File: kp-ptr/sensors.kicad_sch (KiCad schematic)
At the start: 3 parts

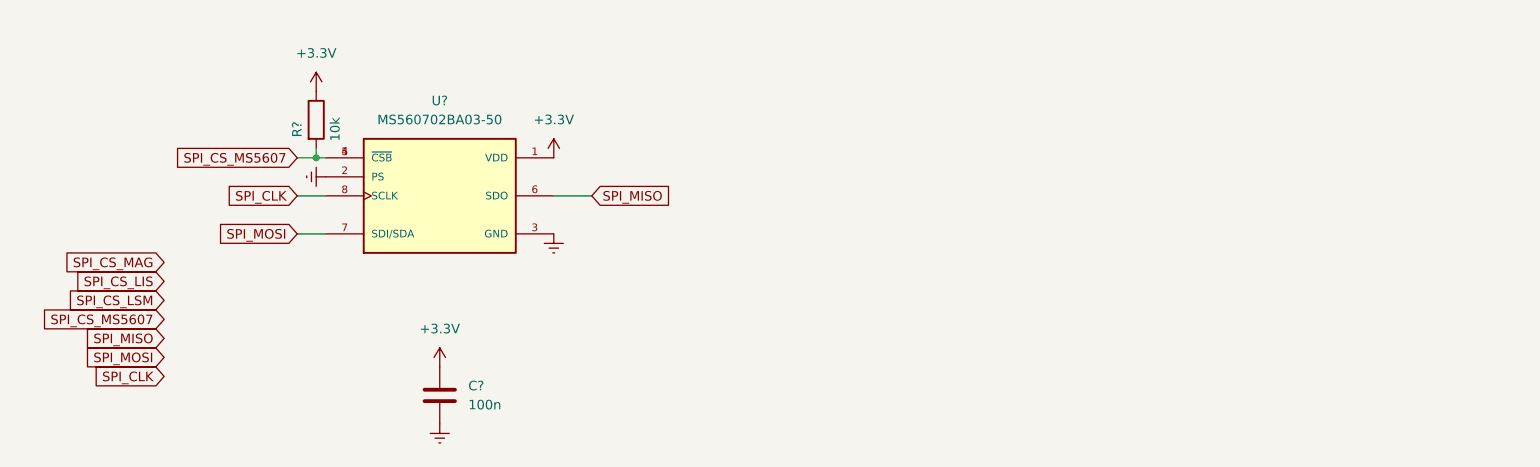
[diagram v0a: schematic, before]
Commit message: LIS + SDCARD Signed-off-by: kretu <krecik@gmail.com>
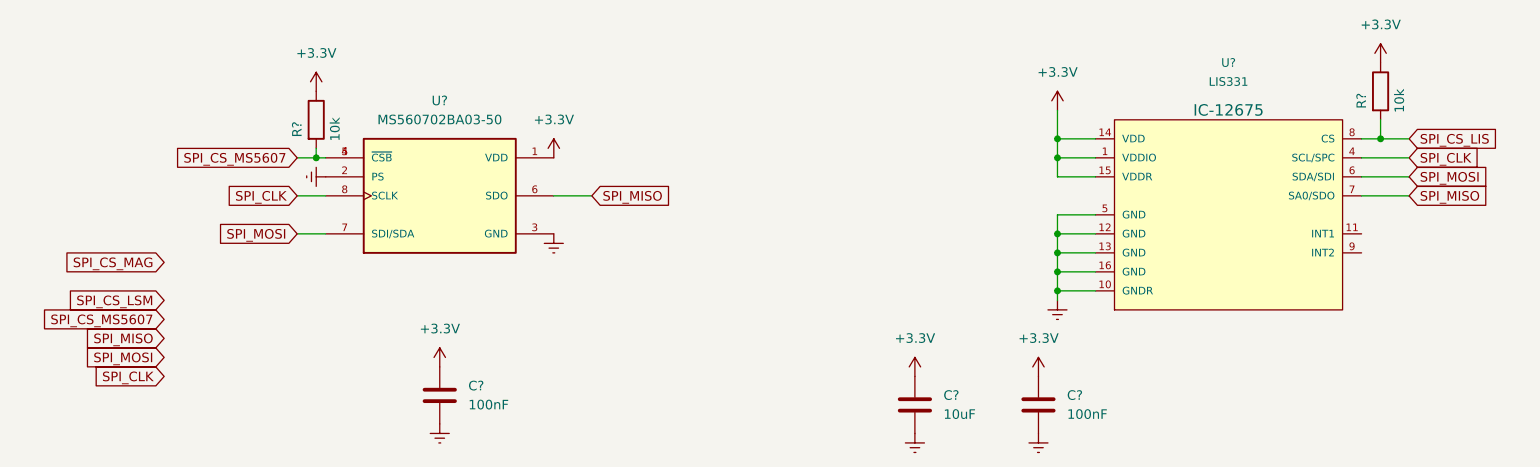
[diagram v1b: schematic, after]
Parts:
- added C?: 10uF, symbol Device:C
- added C?: 100nF, symbol Device:C
- added R?: 10k, symbol Device:R
- added U?: LIS331, LGA-16-3X3, symbol KP-PTR_lib:LIS331
- C?: value 100n -> 100nF
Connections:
- net +3V3: now also C?.1, C?.1, R?.1, U?.1 (VDDIO), U?.14 (VDD), U?.15 (VDDR)
- net Earth: now also C?.2, C?.2, U?.10 (GNDR), U?.12 (GND), U?.13 (GND), U?.16 (GND), U?.5 (GND)
- net SPI_CLK: now also U?.4 (SCL/SPC)
- net SPI_CS_LIS: now also R?.2, U?.8 (CS)
- net SPI_MISO: now also U?.7 (SA0/SDO)
- net SPI_MOSI: now also U?.6 (SDA/SDI)
